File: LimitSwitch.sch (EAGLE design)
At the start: 3 parts, among them X1 53048-02

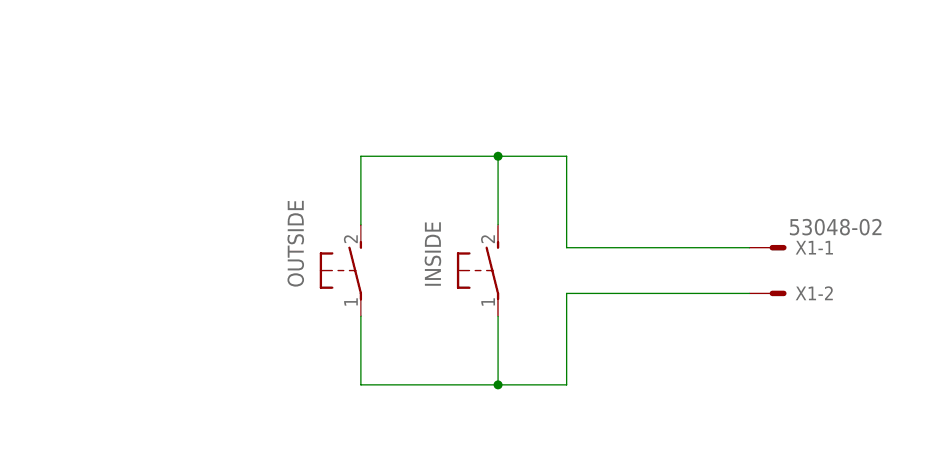
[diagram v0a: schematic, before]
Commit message: sent off an order
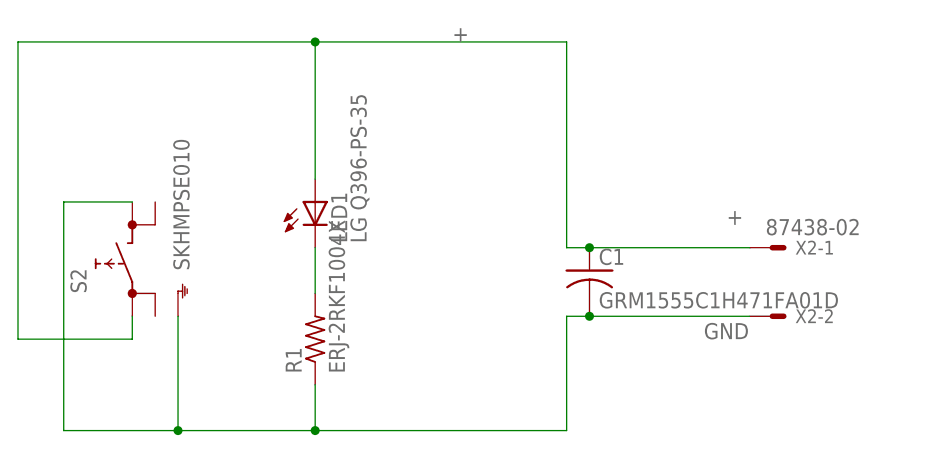
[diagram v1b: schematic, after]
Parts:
- removed INSIDE, OUTSIDE: (no value), switch-omron:31-XX
- removed X1: 53048-02, con-molex:53048-02
- added C1: GRM1555C1H471FA01D, resistor:C-USC0402
- added LED1: LG Q396-PS-35, led:LEDCHIPLED_0603
- added R1: ERJ-2RKF1004X, resistor:R-US_R0402
- added S2: SKHMPSE010, switch:SKHMPSE010
- added X2: 87438-02, con-molex:87438-02
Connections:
- new net N$1: LED1.C, R1.2
- net +: now also C1.1, LED1.A, S2.1.1, X2-1.S; no longer INSIDE.S, OUTSIDE.S, X1-1.S
- net GND: now also C1.2, R1.1, S2.2.1, S2.SH, X2-2.S; no longer INSIDE.P, OUTSIDE.P, X1-2.S
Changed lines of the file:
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@@
 <layer number="97" name="Info" color="7" fill="1" visible="yes" active="yes"/>
 <layer number="98" name="Guide" color="6" fill="1" visible="yes" active="yes"/>
+<layer number="99" name="SpiceOrder" color="5" fill="1" visible="yes" active="yes"/>
 </layers>
 <schematic xreflabel="%F%N/%S.%C%R" xrefpart="/%S.%C%R">
@@
 </classes>
 <parts>
-<part name="INSIDE" library="switch-omron" deviceset="31-XX" device=""/>
-<part name="OUTSIDE" library="switch-omron" deviceset="31-XX" device=""/>
-<part name="X1" library="con-molex" deviceset="53?-02" device="048"/>
+<part name="X2" library="con-molex" deviceset="87438-02" device=""/>
+<part name="S2" library="switch" deviceset="SKHMP*E010" device="" technology="S"/>
+<part name="R1" library="resistor" deviceset="R-US_" device="R0402" value="ERJ-2RKF1004X"/>
+<part name="C1" library="resistor" deviceset="C-US" device="C0402" value="GRM1555C1H471FA01D"/>
+<part name="LED1" library="led" deviceset="LED" device="CHIPLED_0603" value="LG Q396-PS-35"/>
 </parts>
 <sheets>
@@
 </plain>
 <instances>
-<instance part="INSIDE" gate="1" x="66.04" y="53.34" smashed="yes">
-<attribute name="NAME" x="59.69" y="51.435" size="1.778" layer="95" rot="R90"/>
-<attribute name="VALUE" x="62.23" y="56.515" size="1.778" layer="96" rot="R90"/>
-</instance>
-<instance part="OUTSIDE" gate="1" x="50.8" y="53.34" smashed="yes">
-<attribute name="NAME" x="44.45" y="51.435" size="1.778" layer="95" rot="R90"/>
-<attribute name="VALUE" x="46.99" y="56.515" size="1.778" layer="96" rot="R90"/>
-</instance>
-<instance part="X1" gate="-1" x="96.52" y="55.88" smashed="yes">
-<attribute name="NAME" x="99.06" y="55.118" size="1.524" layer="95"/>
-<attribute name="VALUE" x="98.298" y="57.277" size="1.778" layer="96"/>
-</instance>
-<instance part="X1" gate="-2" x="96.52" y="50.8"/>
+<instance part="X2" gate="-1" x="96.52" y="55.88"/>
+<instance part="X2" gate="-2" x="96.52" y="48.26"/>
+<instance part="S2" gate="G$1" x="25.4" y="53.34" rot="R90"/>
+<instance part="R1" gate="G$1" x="45.72" y="45.72" rot="R90"/>
+<instance part="C1" gate="G$1" x="76.2" y="53.34"/>
+<instance part="LED1" gate="G$1" x="45.72" y="60.96"/>
 </instances>
 <busses>
@@
 <net name="+" class="0">
 <segment>
-<wire x1="73.66" y1="55.88" x2="73.66" y2="66.04" width="0.1524" layer="91"/>
-<wire x1="73.66" y1="66.04" x2="66.04" y2="66.04" width="0.1524" layer="91"/>
-<wire x1="66.04" y1="66.04" x2="50.8" y2="66.04" width="0.1524" layer="91"/>
-<pinref part="OUTSIDE" gate="1" pin="S"/>
-<wire x1="50.8" y1="58.42" x2="50.8" y2="66.04" width="0.1524" layer="91"/>
-<pinref part="INSIDE" gate="1" pin="S"/>
-<wire x1="66.04" y1="58.42" x2="66.04" y2="66.04" width="0.1524" layer="91"/>
-<junction x="66.04" y="66.04"/>
-<wire x1="93.98" y1="55.88" x2="73.66" y2="55.88" width="0.1524" layer="91"/>
-<pinref part="X1" gate="-1" pin="S"/>
+<wire x1="93.98" y1="55.88" x2="76.2" y2="55.88" width="0.1524" layer="91"/>
+<label x="91.44" y="58.42" size="1.778" layer="95"/>
+<pinref part="X2" gate="-1" pin="S"/>
+<pinref part="C1" gate="G$1" pin="1"/>
+<wire x1="73.66" y1="78.74" x2="73.66" y2="55.88" width="0.1524" layer="91"/>
+<wire x1="73.66" y1="78.74" x2="45.72" y2="78.74" width="0.1524" layer="91"/>
+<label x="60.96" y="78.74" size="1.778" layer="95"/>
+<wire x1="45.72" y1="78.74" x2="12.7" y2="78.74" width="0.1524" layer="91"/>
+<wire x1="12.7" y1="78.74" x2="12.7" y2="45.72" width="0.1524" layer="91"/>
+<wire x1="12.7" y1="45.72" x2="25.4" y2="45.72" width="0.1524" layer="91"/>
+<pinref part="S2" gate="G$1" pin="1.1"/>
+<wire x1="25.4" y1="45.72" x2="25.4" y2="48.26" width="0.1524" layer="91"/>
+<wire x1="76.2" y1="55.88" x2="73.66" y2="55.88" width="0.1524" layer="91"/>
+<junction x="76.2" y="55.88"/>
+<pinref part="LED1" gate="G$1" pin="A"/>
+<wire x1="45.72" y1="78.74" x2="45.72" y2="63.5" width="0.1524" layer="91"/>
+<junction x="45.72" y="78.74"/>
 </segment>
 </net>
 <net name="GND" class="0">
 <segment>
-<wire x1="73.66" y1="50.8" x2="73.66" y2="40.64" width="0.1524" layer="91"/>
-<wire x1="73.66" y1="40.64" x2="66.04" y2="40.64" width="0.1524" layer="91"/>
-<wire x1="66.04" y1="40.64" x2="50.8" y2="40.64" width="0.1524" layer="91"/>
-<pinref part="OUTSIDE" gate="1" pin="P"/>
-<wire x1="50.8" y1="48.26" x2="50.8" y2="40.64" width="0.1524" layer="91"/>
-<pinref part="INSIDE" gate="1" pin="P"/>
-<wire x1="66.04" y1="48.26" x2="66.04" y2="40.64" width="0.1524" layer="91"/>
-<junction x="66.04" y="40.64"/>
-<wire x1="93.98" y1="50.8" x2="73.66" y2="50.8" width="0.1524" layer="91"/>
-<pinref part="X1" gate="-2" pin="S"/>
+<label x="88.9" y="45.72" size="1.778" layer="95"/>
+<wire x1="73.66" y1="48.26" x2="73.66" y2="35.56" width="0.1524" layer="91"/>
+<pinref part="S2" gate="G$1" pin="SH"/>
+<wire x1="30.48" y1="48.26" x2="30.48" y2="35.56" width="0.1524" layer="91"/>
+<wire x1="30.48" y1="35.56" x2="45.72" y2="35.56" width="0.1524" layer="91"/>
+<junction x="30.48" y="35.56"/>
+<pinref part="X2" gate="-2" pin="S"/>
+<wire x1="45.72" y1="35.56" x2="73.66" y2="35.56" width="0.1524" layer="91"/>
+<wire x1="73.66" y1="48.26" x2="76.2" y2="48.26" width="0.1524" layer="91"/>
+<pinref part="S2" gate="G$1" pin="2.1"/>
+<wire x1="76.2" y1="48.26" x2="93.98" y2="48.26" width="0.1524" layer="91"/>
+<wire x1="25.4" y1="60.96" x2="17.78" y2="60.96" width="0.1524" layer="91"/>
+<wire x1="17.78" y1="60.96" x2="17.78" y2="35.56" width="0.1524" layer="91"/>
+<wire x1="17.78" y1="35.56" x2="30.48" y2="35.56" width="0.1524" layer="91"/>
+<pinref part="C1" gate="G$1" pin="2"/>
+<junction x="76.2" y="48.26"/>
+<pinref part="R1" gate="G$1" pin="1"/>
+<wire x1="45.72" y1="40.64" x2="45.72" y2="35.56" width="0.1524" layer="91"/>
+<junction x="45.72" y="35.56"/>
 </segment>
 </net>
+<net name="N$1" class="0">
+<segment>
+<pinref part="LED1" gate="G$1" pin="C"/>
+<pinref part="R1" gate="G$1" pin="2"/>
+<wire x1="45.72" y1="55.88" x2="45.72" y2="50.8" width="0.1524" layer="91"/>
+</segment>
+</net>
